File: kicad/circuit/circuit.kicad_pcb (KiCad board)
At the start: 2 copper layers, 49.7 x 53.1 mm, 24 parts, among them J1 4X4 Matrix, J1.1 2X2 Matrix A, J1.1.1 Button 1, J1.1.2 Button 2, J1.1.3 Button 5, J1.1.4 Button 6, J1.2 2X2 Matrix B, J1.2.1 Button 3, J1.2.2 Button 4, J1.3 2X2 Matrix C, J1.4 2X2 Matrix D, J2 AVR-ISP, J3 I2C, J4 RJ45, J5 Joystick, U1 ATmega328P-P, Y1 Crystal

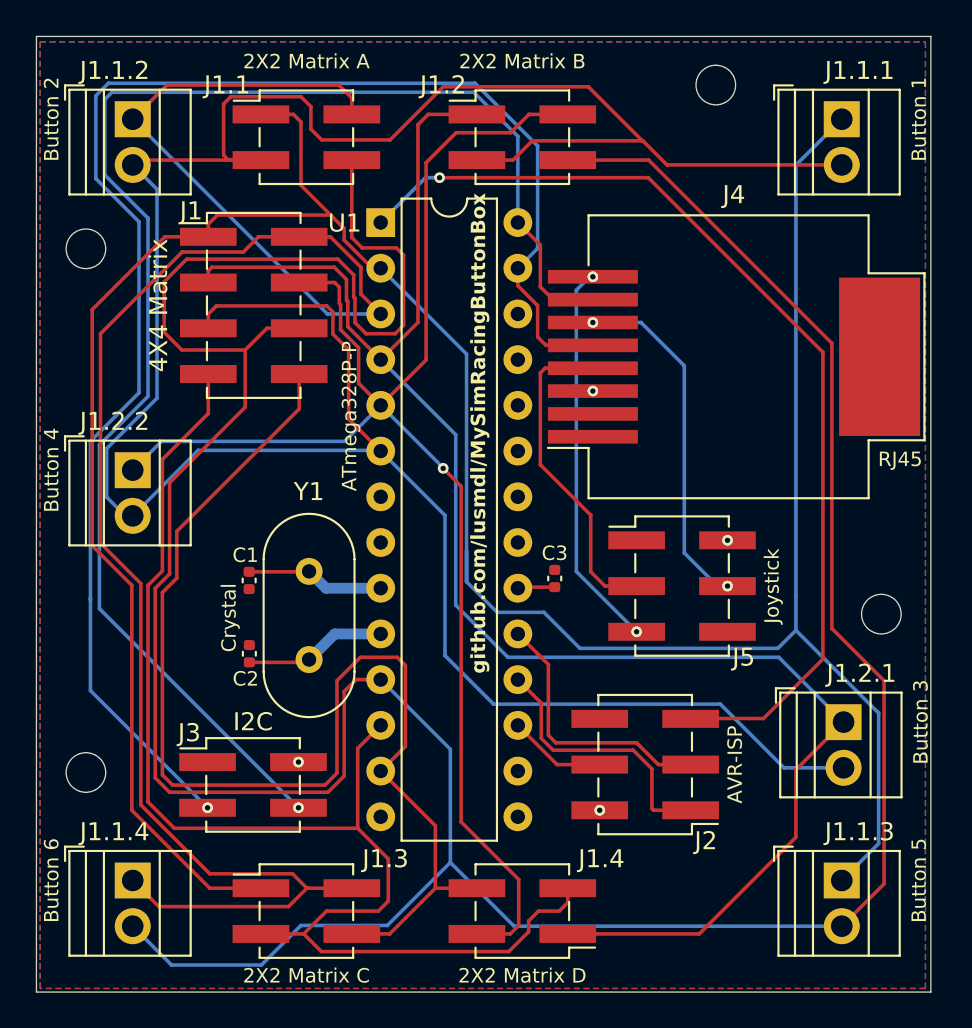
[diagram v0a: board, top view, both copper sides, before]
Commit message: update pcb and documentation
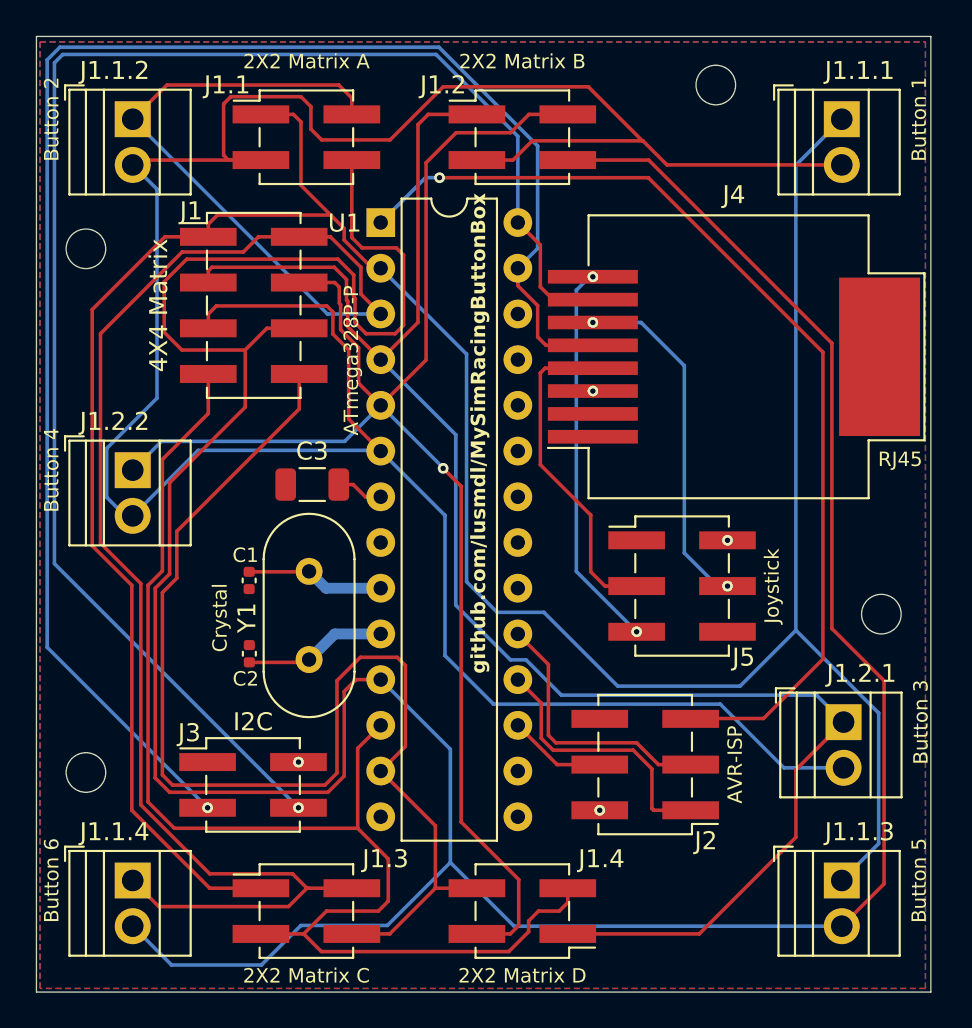
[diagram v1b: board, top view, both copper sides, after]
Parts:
- C3: value 100 µF -> 10 µF; footprint Capacitor_SMD:C_0402_1005Metric -> Capacitor_SMD:C_1206_3216Metric
- moved C3 14.5 mm to (225.3, 67.3), turned to 0 degrees
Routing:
- net /SCL: track 82.3 -> 86.9 mm
- net /SDA: track 85.5 -> 89.9 mm
- net +5V: track 2.07 -> 2.61 mm
